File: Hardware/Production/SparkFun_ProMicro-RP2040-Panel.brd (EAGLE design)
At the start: 132.1 x 140 mm, 1611 parts, among them J1 Qwiic, J12 USB Female Type C Connector, J13 Qwiic, J16 USB Female Type C Connector, J17 Qwiic, J2 Qwiic, J20 USB Female Type C Connector, J21 Qwiic, J24 USB Female Type C Connector, J25 Qwiic, J28 USB Female Type C Connector, J29 Qwiic, J32 USB Female Type C Connector, J33 Qwiic, J36 USB Female Type C Connector, J37 Qwiic, J40 USB Female Type C Connector, J41 Qwiic, J44 USB Female Type C Connector, J45 Qwiic, J48 USB Female Type C Connector, J49 Qwiic, J5 USB Female Type C Connector, J52 USB Female Type C Connector, J53 Qwiic, J56 USB Female Type C Connector, J57 Qwiic, J60 USB Female Type C Connector, J8 USB Female Type C Connector, J9 Qwiic, U1 3.3V, U10 RP2040, U11 W25QXX128MBIT, U12 WS2812-2020, U13 3.3V, U14 RP2040, U15 W25QXX128MBIT, U16 WS2812-2020, U17 3.3V, U18 RP2040, U19 W25QXX128MBIT, U2 RP2040, U20 WS2812-2020, U21 3.3V, U22 RP2040, U23 W25QXX128MBIT, U24 WS2812-2020, U25 3.3V, U26 RP2040, U27 W25QXX128MBIT, U28 WS2812-2020, U29 3.3V, U3 WS2812-2020, U30 RP2040, U31 W25QXX128MBIT, U32 WS2812-2020, U33 3.3V, U34 RP2040, U35 W25QXX128MBIT, U36 WS2812-2020, U37 3.3V, U38 RP2040, U39 W25QXX128MBIT, U4 W25QXX128MBIT, U40 WS2812-2020, U41 3.3V, U42 RP2040, U43 W25QXX128MBIT, U44 WS2812-2020, U45 3.3V, U46 RP2040, U47 W25QXX128MBIT, U48 WS2812-2020, U49 3.3V, U5 3.3V, U50 RP2040, U51 W25QXX128MBIT, U52 WS2812-2020, U53 3.3V, U54 RP2040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

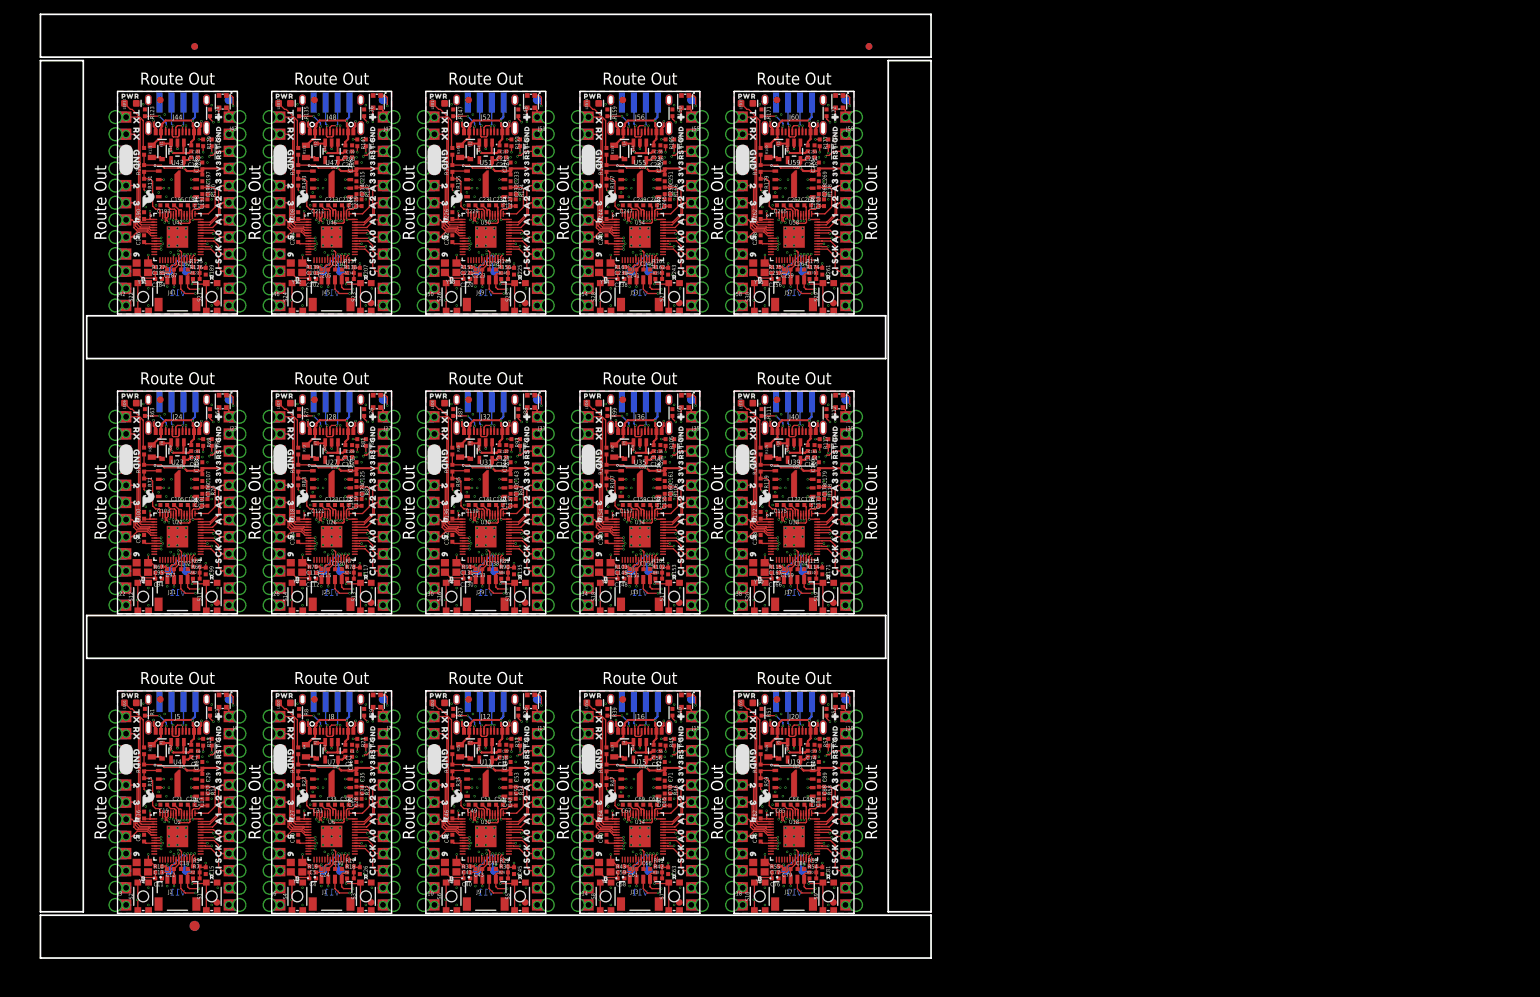
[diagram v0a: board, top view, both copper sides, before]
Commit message: New panel
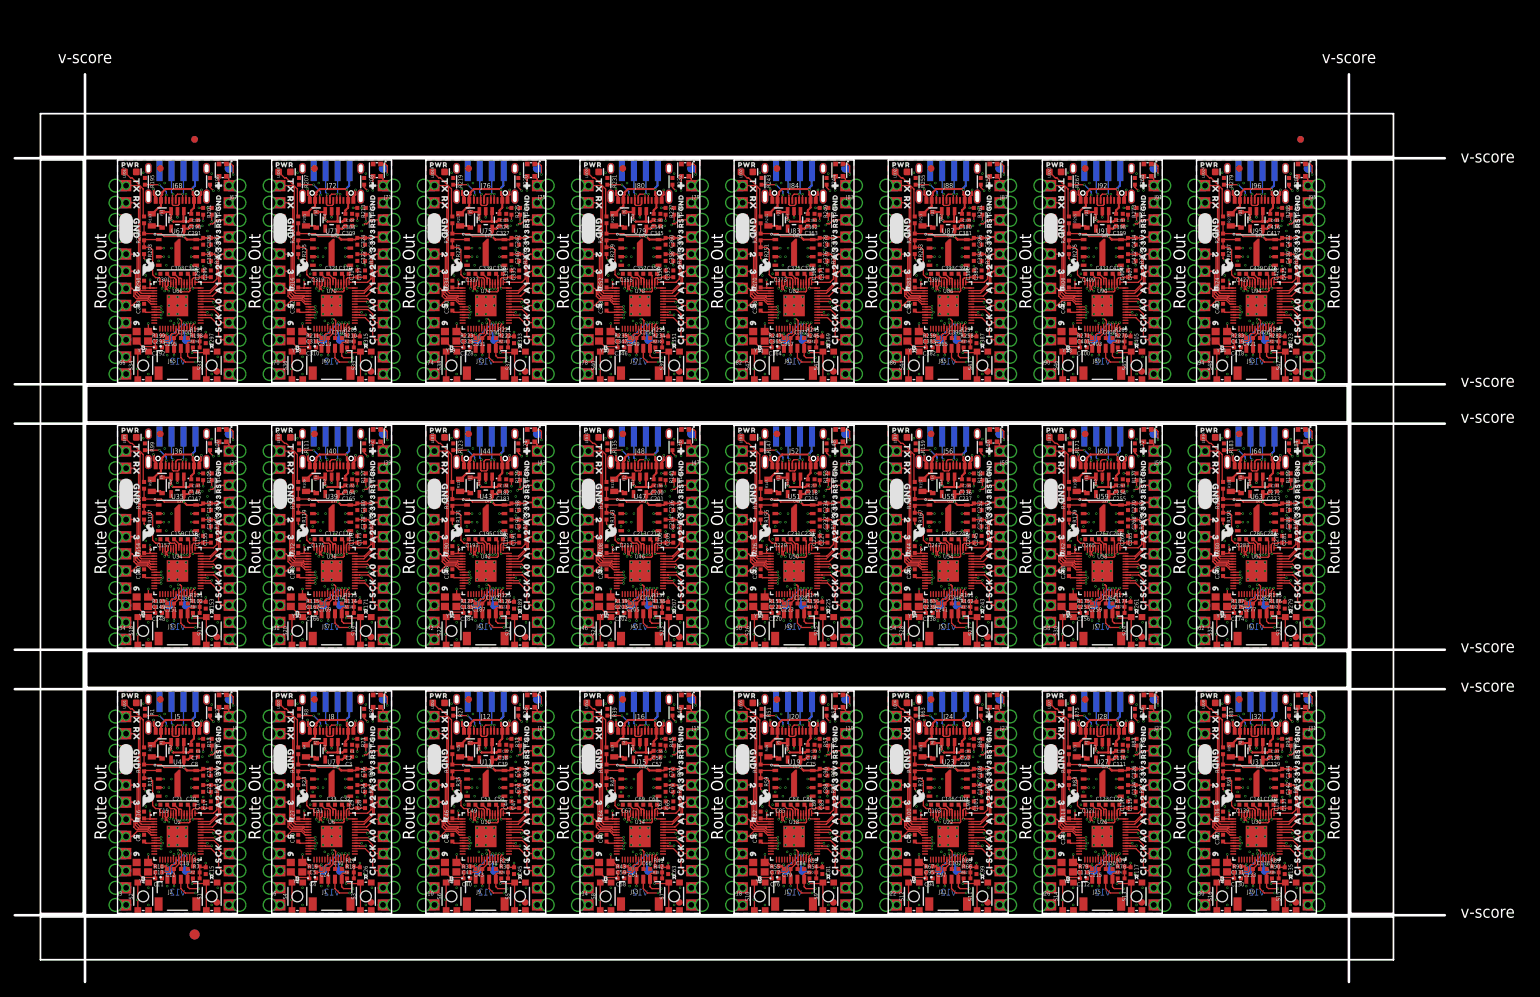
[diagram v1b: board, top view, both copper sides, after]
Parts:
- added C271, C289, C307, C325, C343, C361, C379, C397, C415: 1.0uF, SparkFun-Capacitors:0402-TIGHT
- added C272, C273, C290, C291, C308, C309, C326, C327, C344, C345, C362, C363, C380, C381, C398, C399, C416, C417: 10uF, SparkFun-Capacitors:0402-TIGHT
- added C274, C275, C292, C293, C310, C311, C328, C329, C346, C347, C364, C365, C382, C383, C400, C401, C418, C419: 15pF, SparkFun-Capacitors:0402-TIGHT
- added C276, C277, C278, C279, C280, C281, C282, C283, C287, C294, C295, C296, C297, C298, C299, C300, C301, C305, C312, C313, C314, C315, C316, C317, C318, C319, C323, C330, C331, C332, C333, C334, C335, C336, C337, C341, C348, C349, C350, C351, C352, C353, C354, C355, C359, C366, C367, C368, C369, C370, C371, C372, C373, C377, C384, C385, C386, C387, C388, C389, C390, C391, C395, C402, C403, C404, C405, C406, C407, C408, C409, C413, C420, C421, C422, C423, C424, C425, C426, C427, C431: 0.1uF, SparkFun-Capacitors:0402-TIGHT
- added C284, C285, C286, C288, C302, C303, C304, C306, C320, C321, C322, C324, C338, C339, C340, C342, C356, C357, C358, C360, C374, C375, C376, C378, C392, C393, C394, C396, C410, C411, C412, C414, C428, C429, C430, C432: 2.2uF, SparkFun-Capacitors:0402-TIGHT
- added D16, D17, D18, D19, D20, D21, D22, D23, D24: 3A/10V/280mV, SparkFun-DiscreteSemi:SOD-323
- added F16, F17, F18, F19, F20, F21, F22, F23, F24: 6V 0.5A, SparkFun-Fuses:0805
- added J61, J65, J69, J73, J77, J81, J85, J89, J93: Qwiic, SparkFun-Connectors:JST04_1MM_RA
- added J62, J63, J66, J67, J70, J71, J74, J75, J78, J79, J82, J83, J86, J87, J90, J91, J94, J95: (no value), Castellated:1X12_CASTELLATED
- added J64, J68, J72, J76, J80, J84, J88, J92, J96: USB Female Type C Connector, SparkFun-Connectors:USB-C-16P_4LAYER-PADS
- added JP46, JP47, JP49, JP50, JP52, JP53, JP55, JP56, JP58, JP59, JP61, JP62, JP64, JP65, JP67, JP68, JP70, JP71: FIDUCIAL1X2, SparkFun-Aesthetics:FIDUCIAL-1X2
- added JP48, JP51, JP54, JP57, JP60, JP63, JP66, JP69, JP72: USB_SOLDER_PADS, SparkFun-Connectors:USB-SOLDER-PADS
- added LED16, LED17, LED18, LED19, LED20, LED21, LED22, LED23, LED24: RED, SparkFun-LED:LED-0603
- added LOGO46, LOGO49, LOGO52, LOGO55, LOGO58, LOGO61, LOGO64, LOGO67, LOGO70: SFE_LOGO_NAME_FLAME.1_INCH, SparkFun-Aesthetics:SFE_LOGO_NAME_FLAME_.1
- added LOGO47, LOGO50, LOGO53, LOGO56, LOGO59, LOGO62, LOGO65, LOGO68, LOGO71: QWIIC_LOGO_6MM, SparkFun-Aesthetics:QWIIC_6MM
- added LOGO48, LOGO51, LOGO54, LOGO57, LOGO60, LOGO63, LOGO66, LOGO69, LOGO72: SFE_LOGO_FLAME.1_INCH, SparkFun-Aesthetics:SFE_LOGO_FLAME_.1
- added R181, R187, R191, R193, R199, R203, R205, R211, R215, R217, R223, R227, R229, R235, R239, R241, R247, R251, R253, R259, R263, R265, R271, R275, R277, R283, R287: 1k, SparkFun-Resistors:0402-TIGHT
- added R182, R192, R194, R204, R206, R216, R218, R228, R230, R240, R242, R252, R254, R264, R266, R276, R278, R288: 10k, SparkFun-Resistors:0402-TIGHT
- added R183, R184, R195, R196, R207, R208, R219, R220, R231, R232, R243, R244, R255, R256, R267, R268, R279, R280: 5.1k, SparkFun-Resistors:0402-TIGHT
- added R185, R186, R197, R198, R209, R210, R221, R222, R233, R234, R245, R246, R257, R258, R269, R270, R281, R282: 2.2k, SparkFun-Resistors:0402-TIGHT
- added R188, R189, R200, R201, R212, R213, R224, R225, R236, R237, R248, R249, R260, R261, R272, R273, R284, R285: 27, SparkFun-Resistors:0402-TIGHT
- added R190, R202, R214, R226, R238, R250, R262, R274, R286: 200, SparkFun-Resistors:0402-TIGHT
- added S31, S33, S35, S37, S39, S41, S43, S45, S47: Reset, SparkFun-Switches:TACTILE_SWITCH_SMD_4.6X2.8MM
- added S32, S34, S36, S38, S40, S42, S44, S46, S48: Boot, SparkFun-Switches:TACTILE_SWITCH_SMD_4.6X2.8MM
- added TP46, TP47, TP48, TP49, TP50, TP51, TP52, TP53, TP54, TP55, TP56, TP57, TP58, TP59, TP60, TP61, TP62, TP63, TP64, TP65, TP66, TP67, TP68, TP69, TP70, TP71, TP72: (no value), SparkFun-Connectors:PAD.03X.05
- added U$1000, U$1030, U$1054, U$1084, U$1108, U$1138, U$1162, U$1192, U$1216, U$1246, U$1270, U$814, U$838, U$868, U$892, U$922, U$946, U$976: (no value), output:A21
- added U$1001, U$1031, U$1055, U$1085, U$1109, U$1139, U$1163, U$1193, U$1217, U$1247, U$1271, U$815, U$839, U$869, U$893, U$923, U$947, U$977: (no value), output:A32
- added U$1002, U$1045, U$1056, U$1099, U$1110, U$1153, U$1164, U$1207, U$1218, U$1261, U$1272, U$829, U$840, U$883, U$894, U$937, U$948, U$991: (no value), output:TX0
- added U$1003, U$1044, U$1057, U$1098, U$1111, U$1152, U$1165, U$1206, U$1219, U$1260, U$1273, U$828, U$841, U$882, U$895, U$936, U$949, U$990: (no value), output:RX1
- added U$1004, U$1017, U$1043, U$1058, U$1071, U$1097, U$1112, U$1125, U$1151, U$1166, U$1179, U$1205, U$1220, U$1233, U$1259, U$1274, U$1287, U$827, U$842, U$855, U$881, U$896, U$909, U$935, U$950, U$963, U$989: (no value), output:GND2
- added U$1005, U$1035, U$1059, U$1089, U$1113, U$1143, U$1167, U$1197, U$1221, U$1251, U$1275, U$819, U$843, U$873, U$897, U$927, U$951, U$981: (no value), output:20
- added U$1006, U$1036, U$1060, U$1090, U$1114, U$1144, U$1168, U$1198, U$1222, U$1252, U$1276, U$820, U$844, U$874, U$898, U$928, U$952, U$982: (no value), output:31
- added U$1007, U$1037, U$1061, U$1091, U$1115, U$1145, U$1169, U$1199, U$1223, U$1253, U$1277, U$821, U$845, U$875, U$899, U$929, U$953, U$983: (no value), output:42
- added U$1008, U$1038, U$1062, U$1092, U$1116, U$1146, U$1170, U$1200, U$1224, U$1254, U$1278, U$822, U$846, U$876, U$900, U$930, U$954, U$984: (no value), output:53
- added U$1009, U$1039, U$1063, U$1093, U$1117, U$1147, U$1171, U$1201, U$1225, U$1255, U$1279, U$823, U$847, U$877, U$901, U$931, U$955, U$985: (no value), output:64
- added U$1010, U$1064, U$1118, U$1172, U$1226, U$1280, U$848, U$902, U$956: (no value), output:D#1
- added U$1011, U$1065, U$1119, U$1173, U$1227, U$1281, U$849, U$903, U$957: (no value), output:D#2
- added U$1012, U$1066, U$1120, U$1174, U$1228, U$1282, U$850, U$904, U$958: (no value), output:G0
- added U$1013, U$1067, U$1121, U$1175, U$1229, U$1283, U$851, U$905, U$959: (no value), output:V3
- added U$1014, U$1068, U$1122, U$1176, U$1230, U$1284, U$852, U$906, U$960: (no value), output:210
- added U$1015, U$1069, U$1123, U$1177, U$1231, U$1285, U$853, U$907, U$961: (no value), output:#RST#0
- added U$1016, U$1070, U$1124, U$1178, U$1232, U$1286, U$854, U$908, U$962: (no value), output:3V3_0
- added U$1018, U$1072, U$1126, U$1180, U$1234, U$1288, U$856, U$910, U$964: (no value), output:RAW0
- added U$1019, U$1073, U$1127, U$1181, U$1235, U$1289, U$857, U$911, U$965: (no value), output:B0
- added U$1020, U$1074, U$1128, U$1182, U$1236, U$1290, U$858, U$912, U$966: (no value), output:R0
- added U$1021, U$1075, U$1129, U$1183, U$1237, U$1291, U$859, U$913, U$967: (no value), output:#0
- added U$1022, U$1076, U$1130, U$1184, U$1238, U$1292, U$860, U$914, U$968: (no value), output:PRO_MICRO0
- added U$1023, U$1077, U$1131, U$1185, U$1239, U$1293, U$861, U$915, U$969: (no value), output:RP20401
- added U$1024, U$1078, U$1132, U$1186, U$1240, U$1294, U$862, U$916, U$970: (no value), output:C0
- added U$1025, U$1079, U$1133, U$1187, U$1241, U$1295, U$863, U$917, U$971: (no value), output:D1
- added U$1026, U$1080, U$1134, U$1188, U$1242, U$1296, U$864, U$918, U$972: (no value), output:DO0
- added U$1027, U$1081, U$1135, U$1189, U$1243, U$811, U$865, U$919, U$973: OSHW-LOGOMINI, SparkFun-Aesthetics:OSHW-LOGO-MINI
- added U$1028, U$1052, U$1082, U$1106, U$1136, U$1160, U$1190, U$1214, U$1244, U$1268, U$812, U$836, U$866, U$890, U$920, U$944, U$974, U$998: (no value), output:A00
- added U$1029, U$1053, U$1083, U$1107, U$1137, U$1161, U$1191, U$1215, U$1245, U$1269, U$813, U$837, U$867, U$891, U$921, U$945, U$975, U$999: (no value), output:A10
- added U$1032, U$1050, U$1086, U$1104, U$1140, U$1158, U$1194, U$1212, U$1248, U$1266, U$816, U$834, U$870, U$888, U$924, U$942, U$978, U$996: (no value), output:CI4
- added U$1033, U$1087, U$1141, U$1195, U$1249, U$817, U$871, U$925, U$979: (no value), output:CO5
- added U$1034, U$1051, U$1088, U$1105, U$1142, U$1159, U$1196, U$1213, U$1250, U$1267, U$818, U$835, U$872, U$889, U$926, U$943, U$980, U$997: (no value), output:SCK3
- added U$1040, U$1094, U$1148, U$1202, U$1256, U$824, U$878, U$932, U$986: (no value), output:#RST#1
- added U$1041, U$1095, U$1149, U$1203, U$1257, U$825, U$879, U$933, U$987: (no value), output:3V30
- added U$1042, U$1096, U$1150, U$1204, U$1258, U$826, U$880, U$934, U$988: (no value), output:PWR0
- added U$1046, U$1100, U$1154, U$1208, U$1262, U$830, U$884, U$938, U$992: (no value), output:GND_0
- added U$1047, U$1101, U$1155, U$1209, U$1263, U$831, U$885, U$939, U$993: (no value), output:70
- added U$1048, U$1102, U$1156, U$1210, U$1264, U$832, U$886, U$940, U$994: (no value), output:81
- added U$1049, U$1103, U$1157, U$1211, U$1265, U$833, U$887, U$941, U$995: (no value), output:92
- added U61, U65, U69, U73, U77, U81, U85, U89, U93: 3.3V, SparkFun-IC-Power:SOT23-5
- added U62, U66, U70, U74, U78, U82, U86, U90, U94: RP2040, RP2040:QFN-56
- added U63, U67, U71, U75, U79, U83, U87, U91, U95: W25QXX128MBIT, SparkFun-IC-Memory:WSON-8-6X5-SKINNY_CENTERPAD
- added U64, U68, U72, U76, U80, U84, U88, U92, U96: WS2812-2020, SparkFun-LED:WS2812-2020
- added Y16, Y17, Y18, Y19, Y20, Y21, Y22, Y23, Y24: 12MHz, SparkFun-Clocks:CRYSTAL-SMD-2X2.5MM
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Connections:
- new net !RESET!15: J63.3, J63.3B, R182.1, S31.3, S31.4, U62.26
- new net !RESET!16: J67.3, J67.3B, R194.1, S33.3, S33.4, U66.26
- new net !RESET!17: J71.3, J71.3B, R206.1, S35.3, S35.4, U70.26
- new net !RESET!18: J75.3, J75.3B, R218.1, S37.3, S37.4, U74.26
- new net !RESET!19: J79.3, J79.3B, R230.1, S39.3, S39.4, U78.26
- new net !RESET!20: J83.3, J83.3B, R242.1, S41.3, S41.4, U82.26
- new net !RESET!21: J87.3, J87.3B, R254.1, S43.3, S43.4, U86.26
- new net !RESET!22: J91.3, J91.3B, R266.1, S45.3, S45.4, U90.26
- new net !RESET!23: J95.3, J95.3B, R278.1, S47.3, S47.4, U94.26
- new net 0/TX15: J62.12, J62.12B, U62.2
- new net 0/TX16: J66.12, J66.12B, U66.2
- new net 0/TX17: J70.12, J70.12B, U70.2
- new net 0/TX18: J74.12, J74.12B, U74.2
- new net 0/TX19: J78.12, J78.12B, U78.2
- new net 0/TX20: J82.12, J82.12B, U82.2
- new net 0/TX21: J86.12, J86.12B, U86.2
- new net 0/TX22: J90.12, J90.12B, U90.2
- new net 0/TX23: J94.12, J94.12B, U94.2
- new net 1.1V15: C282.1, C283.1, C284.1, U62.23, U62.45, U62.50
- new net 1.1V16: C300.1, C301.1, C302.1, U66.23, U66.45, U66.50
- new net 1.1V17: C318.1, C319.1, C320.1, U70.23, U70.45, U70.50
- new net 1.1V18: C336.1, C337.1, C338.1, U74.23, U74.45, U74.50
- new net 1.1V19: C354.1, C355.1, C356.1, U78.23, U78.45, U78.50
- new net 1.1V20: C372.1, C373.1, C374.1, U82.23, U82.45, U82.50
- new net 1.1V21: C390.1, C391.1, C392.1, U86.23, U86.45, U86.50
- new net 1.1V22: C408.1, C409.1, C410.1, U90.23, U90.45, U90.50
- new net 1.1V23: C426.1, C427.1, C428.1, U94.23, U94.45, U94.50
- new net 1/RX15: J62.11, J62.11B, U62.3
- new net 1/RX16: J66.11, J66.11B, U66.3
- new net 1/RX17: J70.11, J70.11B, U70.3
- new net 1/RX18: J74.11, J74.11B, U74.3
- new net 1/RX19: J78.11, J78.11B, U78.3
- new net 1/RX20: J82.11, J82.11B, U82.3
- new net 1/RX21: J86.11, J86.11B, U86.3
- new net 1/RX22: J90.11, J90.11B, U90.3
- new net 1/RX23: J94.11, J94.11B, U94.3
- new net 100: J66.3, J66.3B, U66.9
- new net 101: J66.8, J66.8B, U66.4
- new net 102: J66.7, J66.7B, U66.5
- new net 103: J70.5, J70.5B, U70.7
- new net 104: J70.6, J70.6B, U70.6
- new net 105: J70.4, J70.4B, U70.8
- new net 106: J70.3, J70.3B, U70.9
- new net 107: J70.8, J70.8B, U70.4
- new net 108: J70.7, J70.7B, U70.5
- new net 109: J74.5, J74.5B, U74.7
- new net 110: J74.6, J74.6B, U74.6
- new net 111: J74.4, J74.4B, U74.8
- new net 112: J74.3, J74.3B, U74.9
- new net 113: J74.8, J74.8B, U74.4
- new net 114: J74.7, J74.7B, U74.5
- new net 115: J78.5, J78.5B, U78.7
- new net 116: J78.6, J78.6B, U78.6
- new net 117: J78.4, J78.4B, U78.8
- new net 118: J78.3, J78.3B, U78.9
- new net 119: J78.8, J78.8B, U78.4
- new net 120: J78.7, J78.7B, U78.5
- new net 121: J82.5, J82.5B, U82.7
- new net 122: J82.6, J82.6B, U82.6
- new net 123: J82.4, J82.4B, U82.8
- new net 124: J82.3, J82.3B, U82.9
- new net 125: J82.8, J82.8B, U82.4
- new net 126: J82.7, J82.7B, U82.5
- new net 127: J86.5, J86.5B, U86.7
- new net 128: J86.6, J86.6B, U86.6
- new net 129: J86.4, J86.4B, U86.8
- new net 130: J86.3, J86.3B, U86.9
- new net 131: J86.8, J86.8B, U86.4
- new net 132: J86.7, J86.7B, U86.5
- new net 133: J90.5, J90.5B, U90.7
- new net 134: J90.6, J90.6B, U90.6
- new net 135: J90.4, J90.4B, U90.8
- new net 136: J90.3, J90.3B, U90.9
- new net 137: J90.8, J90.8B, U90.4
- new net 138: J90.7, J90.7B, U90.5
- new net 139: J94.5, J94.5B, U94.7
- new net 140: J94.6, J94.6B, U94.6
- new net 141: J94.4, J94.4B, U94.8
- new net 142: J94.3, J94.3B, U94.9
- new net 143: J94.8, J94.8B, U94.4
- new net 144: J94.7, J94.7B, U94.5
- new net 16/SDA15: J61.3, R185.1, U62.27
- new net 16/SDA16: J65.3, R197.1, U66.27
- new net 16/SDA17: J69.3, R209.1, U70.27
- new net 16/SDA18: J73.3, R221.1, U74.27
- new net 16/SDA19: J77.3, R233.1, U78.27
- new net 16/SDA20: J81.3, R245.1, U82.27
- new net 16/SDA21: J85.3, R257.1, U86.27
- new net 16/SDA22: J89.3, R269.1, U90.27
- new net 16/SDA23: J93.3, R281.1, U94.27
- new net 17/SCL15: J61.4, R186.1, U62.28
- new net 17/SCL16: J65.4, R198.1, U66.28
- new net 17/SCL17: J69.4, R210.1, U70.28
- new net 17/SCL18: J73.4, R222.1, U74.28
- new net 17/SCL19: J77.4, R234.1, U78.28
- new net 17/SCL20: J81.4, R246.1, U82.28
- new net 17/SCL21: J85.4, R258.1, U86.28
- new net 17/SCL22: J89.4, R270.1, U90.28
- new net 17/SCL23: J93.4, R282.1, U94.28
- new net 20/SPI_CIPO15: J63.10, J63.10B, U62.31
- new net 20/SPI_CIPO16: J67.10, J67.10B, U66.31
- new net 20/SPI_CIPO17: J71.10, J71.10B, U70.31
- new net 20/SPI_CIPO18: J75.10, J75.10B, U74.31
- new net 20/SPI_CIPO19: J79.10, J79.10B, U78.31
- new net 20/SPI_CIPO20: J83.10, J83.10B, U82.31
- new net 20/SPI_CIPO21: J87.10, J87.10B, U86.31
- new net 20/SPI_CIPO22: J91.10, J91.10B, U90.31
- new net 20/SPI_CIPO23: J95.10, J95.10B, U94.31
- new net 21/SPI_!CS!15: J63.12, J63.12B, U62.32
- new net 21/SPI_!CS!16: J67.12, J67.12B, U66.32
- new net 21/SPI_!CS!17: J71.12, J71.12B, U70.32
- new net 21/SPI_!CS!18: J75.12, J75.12B, U74.32
- new net 21/SPI_!CS!19: J79.12, J79.12B, U78.32
- new net 21/SPI_!CS!20: J83.12, J83.12B, U82.32
- new net 21/SPI_!CS!21: J87.12, J87.12B, U86.32
- new net 21/SPI_!CS!22: J91.12, J91.12B, U90.32
- new net 21/SPI_!CS!23: J95.12, J95.12B, U94.32
- new net 22/SPI_SCK15: J63.9, J63.9B, U62.34
- new net 22/SPI_SCK16: J67.9, J67.9B, U66.34
- new net 22/SPI_SCK17: J71.9, J71.9B, U70.34
- new net 22/SPI_SCK18: J75.9, J75.9B, U74.34
- new net 22/SPI_SCK19: J79.9, J79.9B, U78.34
- new net 22/SPI_SCK20: J83.9, J83.9B, U82.34
- new net 22/SPI_SCK21: J87.9, J87.9B, U86.34
- new net 22/SPI_SCK22: J91.9, J91.9B, U90.34
- new net 22/SPI_SCK23: J95.9, J95.9B, U94.34
- new net 23/SPI_COPI15: J63.11, J63.11B, U62.35
- new net 23/SPI_COPI16: J67.11, J67.11B, U66.35
- new net 23/SPI_COPI17: J71.11, J71.11B, U70.35
- new net 23/SPI_COPI18: J75.11, J75.11B, U74.35
- new net 23/SPI_COPI19: J79.11, J79.11B, U78.35
- new net 23/SPI_COPI20: J83.11, J83.11B, U82.35
- new net 23/SPI_COPI21: J87.11, J87.11B, U86.35
- new net 23/SPI_COPI22: J91.11, J91.11B, U90.35
- new net 23/SPI_COPI23: J95.11, J95.11B, U94.35
- new net 25/WS2812-DI15: U62.37, U64.3
- new net 25/WS2812-DI16: U66.37, U68.3
- new net 25/WS2812-DI17: U70.37, U72.3
- new net 25/WS2812-DI18: U74.37, U76.3
- new net 25/WS2812-DI19: U78.37, U80.3
- new net 25/WS2812-DI20: U82.37, U84.3
- new net 25/WS2812-DI21: U86.37, U88.3
- new net 25/WS2812-DI22: U90.37, U92.3
- new net 25/WS2812-DI23: U94.37, U96.3
- new net 3.3V15: C273.2, C276.1, C277.1, C278.1, C279.1, C280.1, C281.1, C285.1, C287.1, C288.1, J61.2, J63.4, J63.4B, R181.2, R182.2, R185.2, R186.2, R190.2, R192.2, U61.5, U62.1, U62.10, U62.22, U62.33, U62.42, U62.44, U62.48, U62.49, U63.8
- new net 3.3V16: C291.2, C294.1, C295.1, C296.1, C297.1, C298.1, C299.1, C303.1, C305.1, C306.1, J65.2, J67.4, J67.4B, R193.2, R194.2, R197.2, R198.2, R202.2, R204.2, U65.5, U66.1, U66.10, U66.22, U66.33, U66.42, U66.44, U66.48, U66.49, U67.8
- new net 3.3V17: C309.2, C312.1, C313.1, C314.1, C315.1, C316.1, C317.1, C321.1, C323.1, C324.1, J69.2, J71.4, J71.4B, R205.2, R206.2, R209.2, R210.2, R214.2, R216.2, U69.5, U70.1, U70.10, U70.22, U70.33, U70.42, U70.44, U70.48, U70.49, U71.8
- new net 3.3V18: C327.2, C330.1, C331.1, C332.1, C333.1, C334.1, C335.1, C339.1, C341.1, C342.1, J73.2, J75.4, J75.4B, R217.2, R218.2, R221.2, R222.2, R226.2, R228.2, U73.5, U74.1, U74.10, U74.22, U74.33, U74.42, U74.44, U74.48, U74.49, U75.8
- new net 3.3V19: C345.2, C348.1, C349.1, C350.1, C351.1, C352.1, C353.1, C357.1, C359.1, C360.1, J77.2, J79.4, J79.4B, R229.2, R230.2, R233.2, R234.2, R238.2, R240.2, U77.5, U78.1, U78.10, U78.22, U78.33, U78.42, U78.44, U78.48, U78.49, U79.8
- new net 3.3V20: C363.2, C366.1, C367.1, C368.1, C369.1, C370.1, C371.1, C375.1, C377.1, C378.1, J81.2, J83.4, J83.4B, R241.2, R242.2, R245.2, R246.2, R250.2, R252.2, U81.5, U82.1, U82.10, U82.22, U82.33, U82.42, U82.44, U82.48, U82.49, U83.8
- new net 3.3V21: C381.2, C384.1, C385.1, C386.1, C387.1, C388.1, C389.1, C393.1, C395.1, C396.1, J85.2, J87.4, J87.4B, R253.2, R254.2, R257.2, R258.2, R262.2, R264.2, U85.5, U86.1, U86.10, U86.22, U86.33, U86.42, U86.44, U86.48, U86.49, U87.8
- new net 3.3V22: C399.2, C402.1, C403.1, C404.1, C405.1, C406.1, C407.1, C411.1, C413.1, C414.1, J89.2, J91.4, J91.4B, R265.2, R266.2, R269.2, R270.2, R274.2, R276.2, U89.5, U90.1, U90.10, U90.22, U90.33, U90.42, U90.44, U90.48, U90.49, U91.8
- new net 3.3V23: C417.2, C420.1, C421.1, C422.1, C423.1, C424.1, C425.1, C429.1, C431.1, C432.1, J93.2, J95.4, J95.4B, R277.2, R278.2, R281.2, R282.2, R286.2, R288.2, U93.5, U94.1, U94.10, U94.22, U94.33, U94.42, U94.44, U94.48, U94.49, U95.8
- new net 8/TX16: J62.2, J62.2B, U62.11
- new net 8/TX17: J66.2, J66.2B, U66.11
- new net 8/TX18: J70.2, J70.2B, U70.11
- new net 8/TX19: J74.2, J74.2B, U74.11
- new net 8/TX20: J78.2, J78.2B, U78.11
- new net 8/TX21: J82.2, J82.2B, U82.11
- new net 8/TX22: J86.2, J86.2B, U86.11
- new net 8/TX23: J90.2, J90.2B, U90.11
- new net 8/TX24: J94.2, J94.2B, U94.11
- new net 9/RX16: J62.1, J62.1B, U62.12
- new net 9/RX17: J66.1, J66.1B, U66.12
- new net 9/RX18: J70.1, J70.1B, U70.12
- new net 9/RX19: J74.1, J74.1B, U74.12
- new net 9/RX20: J78.1, J78.1B, U78.12
- new net 9/RX21: J82.1, J82.1B, U82.12
- new net 9/RX22: J86.1, J86.1B, U86.12
- new net 9/RX23: J90.1, J90.1B, U90.12
- new net 9/RX24: J94.1, J94.1B, U94.12
- new net 91: J62.5, J62.5B, U62.7
- new net 92: J62.6, J62.6B, U62.6
- new net 93: J62.4, J62.4B, U62.8
- new net 94: J62.3, J62.3B, U62.9
- new net 95: J62.8, J62.8B, U62.4
- new net 96: J62.7, J62.7B, U62.5
- new net 97: J66.5, J66.5B, U66.7
- new net 98: J66.6, J66.6B, U66.6
- new net 99: J66.4, J66.4B, U66.8
- new net A60: J63.5, J63.5B, U62.41
- new net A61: J63.6, J63.6B, U62.40
- new net A62: J63.7, J63.7B, U62.39
- new net A63: J63.8, J63.8B, U62.38
- new net A64: J67.5, J67.5B, U66.41
- new net A65: J67.6, J67.6B, U66.40
- new net A66: J67.7, J67.7B, U66.39
- new net A67: J67.8, J67.8B, U66.38
- new net A68: J71.5, J71.5B, U70.41
- new net A69: J71.6, J71.6B, U70.40
- new net A70: J71.7, J71.7B, U70.39
- new net A71: J71.8, J71.8B, U70.38
- new net A72: J75.5, J75.5B, U74.41
- new net A73: J75.6, J75.6B, U74.40
- new net A74: J75.7, J75.7B, U74.39
- new net A75: J75.8, J75.8B, U74.38
- new net A76: J79.5, J79.5B, U78.41
- new net A77: J79.6, J79.6B, U78.40
- new net A78: J79.7, J79.7B, U78.39
- new net A79: J79.8, J79.8B, U78.38
- new net A80: J83.5, J83.5B, U82.41
- new net A81: J83.6, J83.6B, U82.40
- new net A82: J83.7, J83.7B, U82.39
- new net A83: J83.8, J83.8B, U82.38
- new net A84: J87.5, J87.5B, U86.41
- new net A85: J87.6, J87.6B, U86.40
- new net A86: J87.7, J87.7B, U86.39
- new net A87: J87.8, J87.8B, U86.38
- new net A88: J91.5, J91.5B, U90.41
- new net A89: J91.6, J91.6B, U90.40
- new net A90: J91.7, J91.7B, U90.39
- new net A91: J91.8, J91.8B, U90.38
- new net A92: J95.5, J95.5B, U94.41
- new net A93: J95.6, J95.6B, U94.40
- new net A94: J95.7, J95.7B, U94.39
- new net A95: J95.8, J95.8B, U94.38
- new net ADC_VDD15: C286.1, R190.1, U62.43
- new net ADC_VDD16: C304.1, R202.1, U66.43
- new net ADC_VDD17: C322.1, R214.1, U70.43
- new net ADC_VDD18: C340.1, R226.1, U74.43
- new net ADC_VDD19: C358.1, R238.1, U78.43
- new net ADC_VDD20: C376.1, R250.1, U82.43
- new net ADC_VDD21: C394.1, R262.1, U86.43
- new net ADC_VDD22: C412.1, R274.1, U90.43
- new net ADC_VDD23: C430.1, R286.1, U94.43
- new net BOOT15: R191.2, S32.3, S32.4
- new net BOOT16: R203.2, S34.3, S34.4
- new net BOOT17: R215.2, S36.3, S36.4
- new net BOOT18: R227.2, S38.3, S38.4
- new net BOOT19: R239.2, S40.3, S40.4
- new net BOOT20: R251.2, S42.3, S42.4
- new net BOOT21: R263.2, S44.3, S44.4
- new net BOOT22: R275.2, S46.3, S46.4
- new net BOOT23: R287.2, S48.3, S48.4
- new net GND15: C271.1, C272.1, C273.1, C274.1, C275.1, C276.2, C277.2, C278.2, C279.2, C280.2, C281.2, C282.2, C283.2, C284.2, C285.2, C286.2, C287.2, C288.2, J61.1, J62.10, J62.10B, J62.9, J62.9B, J63.2, J63.2B, J64.GND, J64.GND2, JP48.GND, LED16.C, R183.1, R184.1, S31.1, S31.2, S32.1, S32.2, U61.2, U62.19, U62.EPAD, U63.4, U64.2
- new net GND16: C289.1, C290.1, C291.1, C292.1, C293.1, C294.2, C295.2, C296.2, C297.2, C298.2, C299.2, C300.2, C301.2, C302.2, C303.2, C304.2, C305.2, C306.2, J65.1, J66.10, J66.10B, J66.9, J66.9B, J67.2, J67.2B, J68.GND, J68.GND2, JP51.GND, LED17.C, R195.1, R196.1, S33.1, S33.2, S34.1, S34.2, U65.2, U66.19, U66.EPAD, U67.4, U68.2
- new net GND17: C307.1, C308.1, C309.1, C310.1, C311.1, C312.2, C313.2, C314.2, C315.2, C316.2, C317.2, C318.2, C319.2, C320.2, C321.2, C322.2, C323.2, C324.2, J69.1, J70.10, J70.10B, J70.9, J70.9B, J71.2, J71.2B, J72.GND, J72.GND2, JP54.GND, LED18.C, R207.1, R208.1, S35.1, S35.2, S36.1, S36.2, U69.2, U70.19, U70.EPAD, U71.4, U72.2
- new net GND18: C325.1, C326.1, C327.1, C328.1, C329.1, C330.2, C331.2, C332.2, C333.2, C334.2, C335.2, C336.2, C337.2, C338.2, C339.2, C340.2, C341.2, C342.2, J73.1, J74.10, J74.10B, J74.9, J74.9B, J75.2, J75.2B, J76.GND, J76.GND2, JP57.GND, LED19.C, R219.1, R220.1, S37.1, S37.2, S38.1, S38.2, U73.2, U74.19, U74.EPAD, U75.4, U76.2
- new net GND19: C343.1, C344.1, C345.1, C346.1, C347.1, C348.2, C349.2, C350.2, C351.2, C352.2, C353.2, C354.2, C355.2, C356.2, C357.2, C358.2, C359.2, C360.2, J77.1, J78.10, J78.10B, J78.9, J78.9B, J79.2, J79.2B, J80.GND, J80.GND2, JP60.GND, LED20.C, R231.1, R232.1, S39.1, S39.2, S40.1, S40.2, U77.2, U78.19, U78.EPAD, U79.4, U80.2
- new net GND20: C361.1, C362.1, C363.1, C364.1, C365.1, C366.2, C367.2, C368.2, C369.2, C370.2, C371.2, C372.2, C373.2, C374.2, C375.2, C376.2, C377.2, C378.2, J81.1, J82.10, J82.10B, J82.9, J82.9B, J83.2, J83.2B, J84.GND, J84.GND2, JP63.GND, LED21.C, R243.1, R244.1, S41.1, S41.2, S42.1, S42.2, U81.2, U82.19, U82.EPAD, U83.4, U84.2
- new net GND21: C379.1, C380.1, C381.1, C382.1, C383.1, C384.2, C385.2, C386.2, C387.2, C388.2, C389.2, C390.2, C391.2, C392.2, C393.2, C394.2, C395.2, C396.2, J85.1, J86.10, J86.10B, J86.9, J86.9B, J87.2, J87.2B, J88.GND, J88.GND2, JP66.GND, LED22.C, R255.1, R256.1, S43.1, S43.2, S44.1, S44.2, U85.2, U86.19, U86.EPAD, U87.4, U88.2
- new net GND22: C397.1, C398.1, C399.1, C400.1, C401.1, C402.2, C403.2, C404.2, C405.2, C406.2, C407.2, C408.2, C409.2, C410.2, C411.2, C412.2, C413.2, C414.2, J89.1, J90.10, J90.10B, J90.9, J90.9B, J91.2, J91.2B, J92.GND, J92.GND2, JP69.GND, LED23.C, R267.1, R268.1, S45.1, S45.2, S46.1, S46.2, U89.2, U90.19, U90.EPAD, U91.4, U92.2
- new net GND23: C415.1, C416.1, C417.1, C418.1, C419.1, C420.2, C421.2, C422.2, C423.2, C424.2, C425.2, C426.2, C427.2, C428.2, C429.2, C430.2, C431.2, C432.2, J93.1, J94.10, J94.10B, J94.9, J94.9B, J95.2, J95.2B, J96.GND, J96.GND2, JP72.GND, LED24.C, R279.1, R280.1, S47.1, S47.2, S48.1, S48.2, U93.2, U94.19, U94.EPAD, U95.4, U96.2
- new net N$61: LED16.A, R181.1
- new net N$62: J64.A5, R184.2
- new net N$63: J64.B5, R183.2
- new net N$64: TP48.P$1, U64.1
- new net N$65: LED17.A, R193.1
- new net N$66: J68.A5, R196.2
- new net N$67: J68.B5, R195.2
- new net N$68: TP51.P$1, U68.1
- new net N$69: LED18.A, R205.1
- new net N$70: J72.A5, R208.2
- new net N$71: J72.B5, R207.2
- new net N$72: TP54.P$1, U72.1
- new net N$73: LED19.A, R217.1
- new net N$74: J76.A5, R220.2
- new net N$75: J76.B5, R219.2
- new net N$76: TP57.P$1, U76.1
- new net N$77: LED20.A, R229.1
- new net N$78: J80.A5, R232.2
- new net N$79: J80.B5, R231.2
- new net N$80: TP60.P$1, U80.1
- new net N$81: LED21.A, R241.1
- new net N$82: J84.A5, R244.2
- new net N$83: J84.B5, R243.2
- new net N$84: TP63.P$1, U84.1
- new net N$85: LED22.A, R253.1
- new net N$86: J88.A5, R256.2
- new net N$87: J88.B5, R255.2
- new net N$88: TP66.P$1, U88.1
- new net N$89: LED23.A, R265.1
- new net N$90: J92.A5, R268.2
- new net N$91: J92.B5, R267.2
- new net N$92: TP69.P$1, U92.1
- new net N$93: LED24.A, R277.1
- new net N$94: J96.A5, R280.2
- new net N$95: J96.B5, R279.2
- new net N$96: TP72.P$1, U96.1
- new net QSPI-60: U62.53, U63.5
- new net QSPI-61: U62.51, U63.7
- new net QSPI-62: U62.55, U63.2
- new net QSPI-63: U62.54, U63.3
- new net QSPI-64: U66.53, U67.5
- new net QSPI-65: U66.51, U67.7
- new net QSPI-66: U66.55, U67.2
- new net QSPI-67: U66.54, U67.3
- new net QSPI-68: U70.53, U71.5
- new net QSPI-69: U70.51, U71.7
- new net QSPI-70: U70.55, U71.2
- new net QSPI-71: U70.54, U71.3
- new net QSPI-72: U74.53, U75.5
- new net QSPI-73: U74.51, U75.7
- new net QSPI-74: U74.55, U75.2
- new net QSPI-75: U74.54, U75.3
- new net QSPI-76: U78.53, U79.5
- new net QSPI-77: U78.51, U79.7
- new net QSPI-78: U78.55, U79.2
- new net QSPI-79: U78.54, U79.3
- new net QSPI-80: U82.53, U83.5
- new net QSPI-81: U82.51, U83.7
- new net QSPI-82: U82.55, U83.2
- new net QSPI-83: U82.54, U83.3
- new net QSPI-84: U86.53, U87.5
- new net QSPI-85: U86.51, U87.7
- new net QSPI-86: U86.55, U87.2
- new net QSPI-87: U86.54, U87.3
- new net QSPI-88: U90.53, U91.5
- new net QSPI-89: U90.51, U91.7
- new net QSPI-90: U90.55, U91.2
- new net QSPI-91: U90.54, U91.3
- new net QSPI-92: U94.53, U95.5
- new net QSPI-93: U94.51, U95.7
- new net QSPI-94: U94.55, U95.2
- new net QSPI-95: U94.54, U95.3
- new net QSPI-CLK15: U62.52, U63.6
- new net QSPI-CLK16: U66.52, U67.6
- new net QSPI-CLK17: U70.52, U71.6
- new net QSPI-CLK18: U74.52, U75.6
- new net QSPI-CLK19: U78.52, U79.6
- new net QSPI-CLK20: U82.52, U83.6
- new net QSPI-CLK21: U86.52, U87.6
- new net QSPI-CLK22: U90.52, U91.6
- new net QSPI-CLK23: U94.52, U95.6
- new net QSPI-CS15: R191.1, R192.1, U62.56, U63.1
- new net QSPI-CS16: R203.1, R204.1, U66.56, U67.1
- new net QSPI-CS17: R215.1, R216.1, U70.56, U71.1
- new net QSPI-CS18: R227.1, R228.1, U74.56, U75.1
- new net QSPI-CS19: R239.1, R240.1, U78.56, U79.1
- new net QSPI-CS20: R251.1, R252.1, U82.56, U83.1
- new net QSPI-CS21: R263.1, R264.1, U86.56, U87.1
- new net QSPI-CS22: R275.1, R276.1, U90.56, U91.1
- new net QSPI-CS23: R287.1, R288.1, U94.56, U95.1
- new net RAW15: C272.2, D16.C, J63.1, J63.1B, U61.1, U61.3, U64.4
- new net RAW16: C290.2, D17.C, J67.1, J67.1B, U65.1, U65.3, U68.4
- new net RAW17: C308.2, D18.C, J71.1, J71.1B, U69.1, U69.3, U72.4
- new net RAW18: C326.2, D19.C, J75.1, J75.1B, U73.1, U73.3, U76.4
- new net RAW19: C344.2, D20.C, J79.1, J79.1B, U77.1, U77.3, U80.4
- new net RAW20: C362.2, D21.C, J83.1, J83.1B, U81.1, U81.3, U84.4
- new net RAW21: C380.2, D22.C, J87.1, J87.1B, U85.1, U85.3, U88.4
- new net RAW22: C398.2, D23.C, J91.1, J91.1B, U89.1, U89.3, U92.4
- new net RAW23: C416.2, D24.C, J95.1, J95.1B, U93.1, U93.3, U96.4
- new net RP_D+15: J64.A6, J64.B6, JP48.D+, R189.1
- new net RP_D+16: J68.A6, J68.B6, JP51.D+, R201.1
- new net RP_D+17: J72.A6, J72.B6, JP54.D+, R213.1
- new net RP_D+18: J76.A6, J76.B6, JP57.D+, R225.1
- new net RP_D+19: J80.A6, J80.B6, JP60.D+, R237.1
- new net RP_D+20: J84.A6, J84.B6, JP63.D+, R249.1
- new net RP_D+21: J88.A6, J88.B6, JP66.D+, R261.1
- new net RP_D+22: J92.A6, J92.B6, JP69.D+, R273.1
- new net RP_D+23: J96.A6, J96.B6, JP72.D+, R285.1
- new net RP_D-15: J64.A7, J64.B7, JP48.D-, R188.1
- new net RP_D-16: J68.A7, J68.B7, JP51.D-, R200.1
- new net RP_D-17: J72.A7, J72.B7, JP54.D-, R212.1
- new net RP_D-18: J76.A7, J76.B7, JP57.D-, R224.1
- new net RP_D-19: J80.A7, J80.B7, JP60.D-, R236.1
- new net RP_D-20: J84.A7, J84.B7, JP63.D-, R248.1
- new net RP_D-21: J88.A7, J88.B7, JP66.D-, R260.1
- new net RP_D-22: J92.A7, J92.B7, JP69.D-, R272.1
- new net RP_D-23: J96.A7, J96.B7, JP72.D-, R284.1
- new net RP_D1+15: R189.2, U62.47
- new net RP_D1+16: R201.2, U66.47
- new net RP_D1+17: R213.2, U70.47
- new net RP_D1+18: R225.2, U74.47
- new net RP_D1+19: R237.2, U78.47
- new net RP_D1+20: R249.2, U82.47
- new net RP_D1+21: R261.2, U86.47
- new net RP_D1+22: R273.2, U90.47
- new net RP_D1+23: R285.2, U94.47
- new net RP_D1-15: R188.2, U62.46
- new net RP_D1-16: R200.2, U66.46
- new net RP_D1-17: R212.2, U70.46
- new net RP_D1-18: R224.2, U74.46
- new net RP_D1-19: R236.2, U78.46
- new net RP_D1-20: R248.2, U82.46
- new net RP_D1-21: R260.2, U86.46
- new net RP_D1-22: R272.2, U90.46
- new net RP_D1-23: R284.2, U94.46
- new net SWDCK15: TP46.P$1, U62.24
- new net SWDCK16: TP49.P$1, U66.24
- new net SWDCK17: TP52.P$1, U70.24
- new net SWDCK18: TP55.P$1, U74.24
- new net SWDCK19: TP58.P$1, U78.24
- new net SWDCK20: TP61.P$1, U82.24
- new net SWDCK21: TP64.P$1, U86.24
- new net SWDCK22: TP67.P$1, U90.24
- new net SWDCK23: TP70.P$1, U94.24
- new net SWDIO15: TP47.P$1, U62.25
- new net SWDIO16: TP50.P$1, U66.25
- new net SWDIO17: TP53.P$1, U70.25
- new net SWDIO18: TP56.P$1, U74.25
- new net SWDIO19: TP59.P$1, U78.25
- new net SWDIO20: TP62.P$1, U82.25
- new net SWDIO21: TP65.P$1, U86.25
- new net SWDIO22: TP68.P$1, U90.25
- new net SWDIO23: TP71.P$1, U94.25
- new net USB_RAW15: D16.A, F16.2
- new net USB_RAW16: D17.A, F17.2
- new net USB_RAW17: D18.A, F18.2
- new net USB_RAW18: D19.A, F19.2
- new net USB_RAW19: D20.A, F20.2
- new net USB_RAW20: D21.A, F21.2
- new net USB_RAW21: D22.A, F22.2
- new net USB_RAW22: D23.A, F23.2
- new net USB_RAW23: D24.A, F24.2
- new net V_USB15: C271.2, F16.1, J64.VBUS1, J64.VBUS2, JP48.VBUS
- new net V_USB16: C289.2, F17.1, J68.VBUS1, J68.VBUS2, JP51.VBUS
- new net V_USB17: C307.2, F18.1, J72.VBUS1, J72.VBUS2, JP54.VBUS
- new net V_USB18: C325.2, F19.1, J76.VBUS1, J76.VBUS2, JP57.VBUS
- new net V_USB19: C343.2, F20.1, J80.VBUS1, J80.VBUS2, JP60.VBUS
- new net V_USB20: C361.2, F21.1, J84.VBUS1, J84.VBUS2, JP63.VBUS
- new net V_USB21: C379.2, F22.1, J88.VBUS1, J88.VBUS2, JP66.VBUS
- new net V_USB22: C397.2, F23.1, J92.VBUS1, J92.VBUS2, JP69.VBUS
- new net V_USB23: C415.2, F24.1, J96.VBUS1, J96.VBUS2, JP72.VBUS
- new net X16: C275.2, U62.20, Y16.P3
- new net X17: C293.2, U66.20, Y17.P3
- new net X18: C311.2, U70.20, Y18.P3
- new net X19: C329.2, U74.20, Y19.P3
- new net X1A15: R187.2, U62.21
- new net X1A16: R199.2, U66.21
- new net X1A17: R211.2, U70.21
- new net X1A18: R223.2, U74.21
- new net X1A19: R235.2, U78.21
- new net X1A20: R247.2, U82.21
- new net X1A21: R259.2, U86.21
- new net X1A22: R271.2, U90.21
- new net X1A23: R283.2, U94.21
- new net X1B15: C274.2, R187.1, Y16.P1
- new net X1B16: C292.2, R199.1, Y17.P1
- new net X1B17: C310.2, R211.1, Y18.P1
- new net X1B18: C328.2, R223.1, Y19.P1
- new net X1B19: C346.2, R235.1, Y20.P1
- new net X1B20: C364.2, R247.1, Y21.P1
- new net X1B21: C382.2, R259.1, Y22.P1
- new net X1B22: C400.2, R271.1, Y23.P1
- new net X1B23: C418.2, R283.1, Y24.P1
- new net X20: C347.2, U78.20, Y20.P3
- new net X21: C365.2, U82.20, Y21.P3
- new net X22: C383.2, U86.20, Y22.P3
- new net X23: C401.2, U90.20, Y23.P3
- new net X24: C419.2, U94.20, Y24.P3
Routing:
- net 3.3V20: track 0.00 -> 43.5 mm, vias 0 -> 10
- net 3.3V22: track 0.00 -> 43.5 mm, vias 0 -> 10
- net 3.3V21: track 0.00 -> 43.5 mm, vias 0 -> 10
- net 3.3V19: track 0.00 -> 43.5 mm, vias 0 -> 10
- net 3.3V18: track 0.00 -> 43.5 mm, vias 0 -> 10
- net 3.3V17: track 0.00 -> 43.5 mm, vias 0 -> 10
- net 3.3V16: track 0.00 -> 43.5 mm, vias 0 -> 10
- net 3.3V23: track 0.00 -> 43.5 mm, vias 0 -> 10
- net 3.3V15: track 0.00 -> 43.5 mm, vias 0 -> 10
- net !RESET!22: track 0.00 -> 33.0 mm, vias 0 -> 3
- net !RESET!15: track 0.00 -> 33.0 mm, vias 0 -> 3
- net !RESET!16: track 0.00 -> 33.0 mm, vias 0 -> 3
- net !RESET!23: track 0.00 -> 33.0 mm, vias 0 -> 3
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- added copper zone on layer 15, net 3.3V15
- added copper zone on layer 15, net 3.3V16
- added copper zone on layer 15, net 3.3V17
- added copper zone on layer 15, net 3.3V18
- added copper zone on layer 15, net 3.3V19
- added copper zone on layer 15, net 3.3V20
- added copper zone on layer 15, net 3.3V21
- added copper zone on layer 15, net 3.3V22
- added copper zone on layer 15, net 3.3V23
- added copper zone on layer 1, net GND15
- added copper zone on layer 16, net GND15
- added copper zone on layer 2, net GND15
- added copper zone on layer 1, net GND16
- added copper zone on layer 16, net GND16
- added copper zone on layer 2, net GND16
- added copper zone on layer 1, net GND17
- added copper zone on layer 16, net GND17
- added copper zone on layer 2, net GND17
- added copper zone on layer 1, net GND18
- added copper zone on layer 16, net GND18
- added copper zone on layer 2, net GND18
- added copper zone on layer 1, net GND19
- added copper zone on layer 16, net GND19
- added copper zone on layer 2, net GND19
- added copper zone on layer 1, net GND20
- added copper zone on layer 16, net GND20
- added copper zone on layer 2, net GND20
- added copper zone on layer 1, net GND21
- added copper zone on layer 16, net GND21
- added copper zone on layer 2, net GND21
- added copper zone on layer 1, net GND22
- added copper zone on layer 16, net GND22
- added copper zone on layer 2, net GND22
- added copper zone on layer 1, net GND23
- added copper zone on layer 16, net GND23
- added copper zone on layer 2, net GND23
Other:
- board size 132.1 x 140 mm -> 212.1 x 134.6 mm
- board text added: "v-score"
- board text added: "v12"
- board text removed: "v11"
